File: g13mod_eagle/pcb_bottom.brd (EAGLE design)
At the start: 96.4 x 39.8 mm, 42 parts

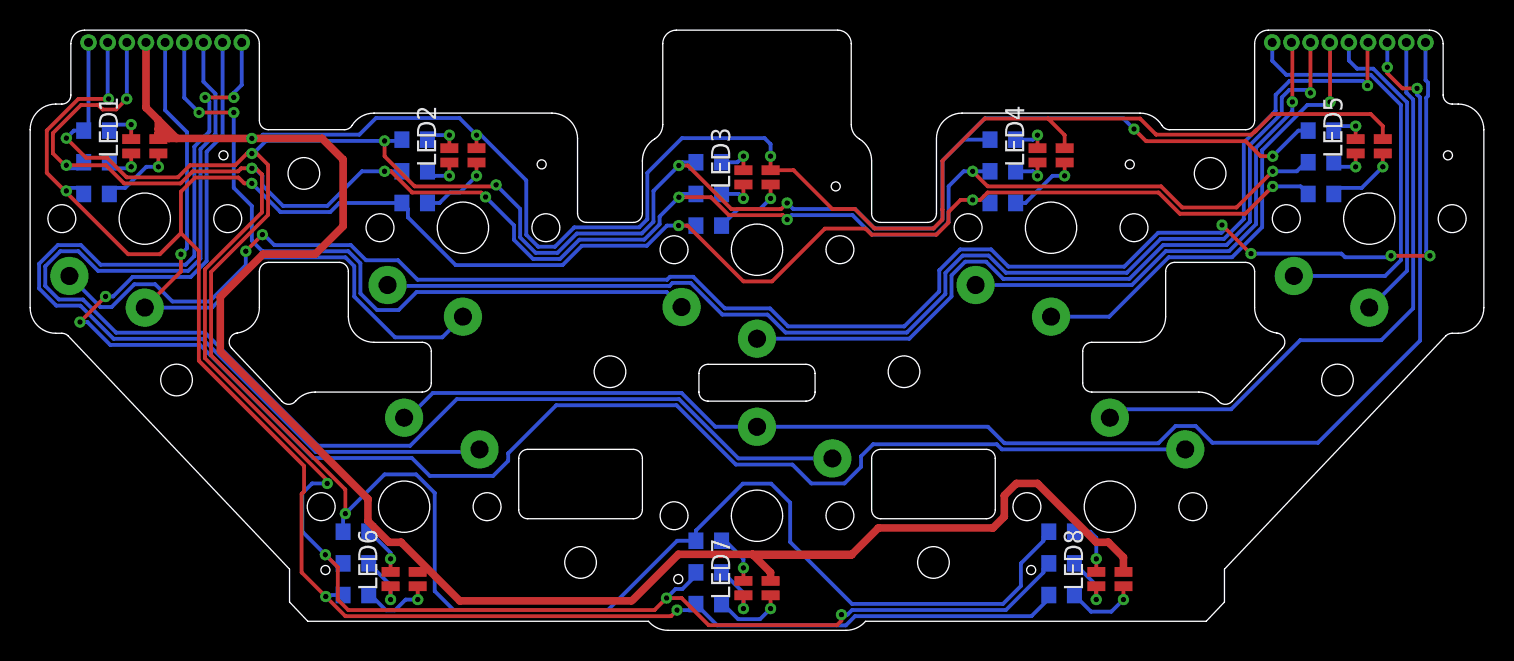
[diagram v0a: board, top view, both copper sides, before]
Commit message: Fix bug
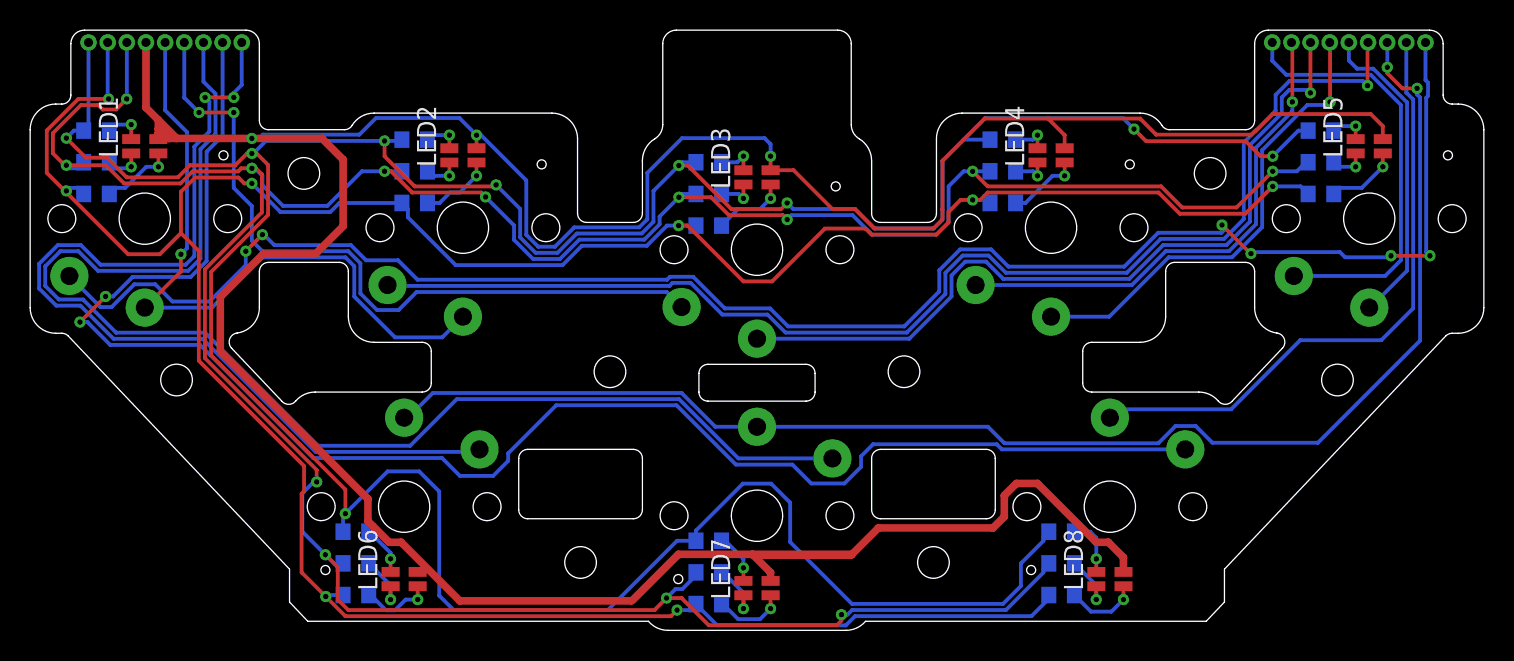
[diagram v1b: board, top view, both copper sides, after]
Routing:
- net G: track 205.7 -> 204.6 mm
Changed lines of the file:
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@@
 <wire x1="-36.2" y1="-1.4700125" x2="-32.4275" y2="2.3024875" width="0.254" layer="1"/>
 <wire x1="-32.4275" y1="2.3024875" x2="-32.4275" y2="5.6275" width="0.254" layer="1"/>
-<wire x1="-27.3" y1="-17.5" x2="-24.7" y2="-14.9" width="0.254" layer="16"/>
-<wire x1="-24.7" y1="-14.9" x2="-22.6" y2="-14.9" width="0.254" layer="16"/>
-<wire x1="-22.6" y1="-14.9" x2="-21.373" y2="-16.127" width="0.254" layer="16"/>
-<wire x1="-21.373" y1="-16.127" x2="-21.373" y2="-22.6395" width="0.254" layer="16"/>
+<wire x1="-27.3" y1="-17.5" x2="-24.5" y2="-14.7" width="0.254" layer="16"/>
+<wire x1="-24.5" y1="-14.7" x2="-22.4" y2="-14.7" width="0.254" layer="16"/>
+<wire x1="-22.4" y1="-14.7" x2="-21.073" y2="-16.027" width="0.254" layer="16"/>
+<wire x1="-21.073" y1="-16.027" x2="-21.073" y2="-22.9395" width="0.254" layer="16"/>
 <wire x1="-9.9" y1="-23.9" x2="-5.3" y2="-19.3" width="0.254" layer="16"/>
 <wire x1="-5.3" y1="-19.3" x2="-4.05" y2="-19.3" width="0.254" layer="16"/>
-<wire x1="-21.373" y1="-22.6395" x2="-20.1125" y2="-23.9" width="0.254" layer="16"/>
+<wire x1="-21.073" y1="-22.9395" x2="-20.1125" y2="-23.9" width="0.254" layer="16"/>
 <wire x1="-20.1125" y1="-23.9" x2="-9.9" y2="-23.9" width="0.254" layer="16"/>
 <wire x1="19.35" y1="-18.7" x2="19" y2="-19.05" width="0.254" layer="16"/>
@@
 <wire x1="28.2" y1="2.8" x2="26.8" y2="4.2" width="0.254" layer="1"/>
 <wire x1="26.8" y1="4.2" x2="15.3" y2="4.2" width="0.254" layer="1"/>
-<wire x1="-28.5" y1="-15.3" x2="-28.5" y2="-15.5" width="0.254" layer="1"/>
-<via x="-28.5" y="-15.5" extent="1-16" drill="0.35"/>
-<wire x1="-28.5" y1="-15.5" x2="-29.5" y2="-15.5" width="0.254" layer="16"/>
+<wire x1="-29.2" y1="-14.6" x2="-29.2" y2="-15.4" width="0.254" layer="1"/>
+<via x="-29.2" y="-15.4" extent="1-16" drill="0.35"/>
+<wire x1="-29.2" y1="-15.4" x2="-29.4" y2="-15.4" width="0.254" layer="16"/>
 <wire x1="-30.152" y1="-16.152" x2="-30.152" y2="-18.698" width="0.254" layer="16"/>
 <wire x1="-30.152" y1="-18.698" x2="-28.625" y2="-20.225" width="0.254" layer="16"/>
-<wire x1="-36.6064" y1="-7.1936" x2="-28.5" y2="-15.3" width="0.254" layer="1"/>
-<wire x1="-29.5" y1="-15.5" x2="-30.152" y2="-16.152" width="0.254" layer="16"/>
+<wire x1="-36.6064" y1="-7.1936" x2="-29.2" y2="-14.6" width="0.254" layer="1"/>
+<wire x1="-29.4" y1="-15.4" x2="-30.152" y2="-16.152" width="0.254" layer="16"/>
 <wire x1="-33.5" y1="5.4" x2="-33.2339" y2="5.4" width="0.254" layer="1"/>
 <wire x1="-33.2339" y1="5.4" x2="-32.8339" y2="5" width="0.254" layer="1"/>
@@
 <wire x1="41.5" y1="7.335" x2="41.5" y2="8.2" width="0.254" layer="1"/>
 <wire x1="34.2" y1="9" x2="33.1" y2="7.9" width="0.254" layer="1"/>
-<wire x1="33" y1="7.8" x2="33.1" y2="7.9" width="0.254" layer="1"/>
 <wire x1="33.1" y1="7.9" x2="33.05636875" y2="7.9" width="0.254" layer="1"/>
 <wire x1="33.05636875" y1="7.9" x2="32.78886875" y2="7.6325" width="0.254" layer="1"/>
@@
 <wire x1="-16.5" y1="-13.5" x2="-16.5" y2="-14" width="0.254" layer="16"/>
 <wire x1="-16.5" y1="-14" x2="-17.5" y2="-15" width="0.254" layer="16"/>
-<wire x1="-21.7" y1="-15" x2="-22.8872" y2="-13.8128" width="0.254" layer="16"/>
+<wire x1="-19.7" y1="-15" x2="-20.8872" y2="-13.8128" width="0.254" layer="16"/>
 <wire x1="-42.8872" y1="-6.3128" x2="-44.4" y2="-4.8" width="0.254" layer="16"/>
 <wire x1="-44.4" y1="-4.8" x2="-44.9" y2="-4.8" width="0.254" layer="16"/>
@@
 <wire x1="-1.403075" y1="-14.2464" x2="-5.336675" y2="-10.3128" width="0.254" layer="16"/>
 <wire x1="-5.336675" y1="-10.3128" x2="-13.3128" y2="-10.3128" width="0.254" layer="16"/>
-<wire x1="-17.5" y1="-15" x2="-21.7" y2="-15" width="0.254" layer="16"/>
-<wire x1="-22.8872" y1="-13.8128" x2="-29.436675" y2="-13.8128" width="0.254" layer="16"/>
+<wire x1="-17.5" y1="-15" x2="-19.7" y2="-15" width="0.254" layer="16"/>
+<wire x1="-20.8872" y1="-13.8128" x2="-29.436675" y2="-13.8128" width="0.254" layer="16"/>
 <wire x1="-29.436675" y1="-13.8128" x2="-36.936675" y2="-6.3128" width="0.254" layer="16"/>
 <wire x1="-36.936675" y1="-6.3128" x2="-42.8872" y2="-6.3128" width="0.254" layer="16"/>
@@
 <wire x1="32.7300875" y1="-0.257075" x2="30.83650625" y2="1.63650625" width="0.254" layer="1"/>
 <via x="32.757075" y="-0.257075" extent="1-16" drill="0.35"/>
-<wire x1="32.757075" y1="-0.257075" x2="38.757075" y2="-0.257075" width="0.254" layer="16"/>
-<wire x1="38.757075" y1="-0.257075" x2="39" y2="-0.5" width="0.254" layer="16"/>
+<wire x1="38.657075" y1="-0.157075" x2="32.857075" y2="-0.157075" width="0.254" layer="16"/>
+<wire x1="32.757075" y1="-0.257075" x2="32.857075" y2="-0.157075" width="0.254" layer="16"/>
+<wire x1="38.657075" y1="-0.157075" x2="39" y2="-0.5" width="0.254" layer="16"/>
 <wire x1="39" y1="-0.5" x2="41.9424" y2="-0.5" width="0.254" layer="16"/>
 <wire x1="41.9424" y1="-0.5" x2="42.0424" y2="-0.4" width="0.254" layer="16"/>
@@
 <via x="-20.4" y="4.9" extent="1-16" drill="0.35"/>
 <wire x1="-20.4" y1="4.9" x2="-20.4" y2="5.785" width="0.254" layer="1"/>
-<wire x1="-20.4" y1="4.9" x2="-20.3936" y2="4.9" width="0.254" layer="16"/>
 </signal>
 <signal name="N$5">
